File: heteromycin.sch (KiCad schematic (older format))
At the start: 0 parts

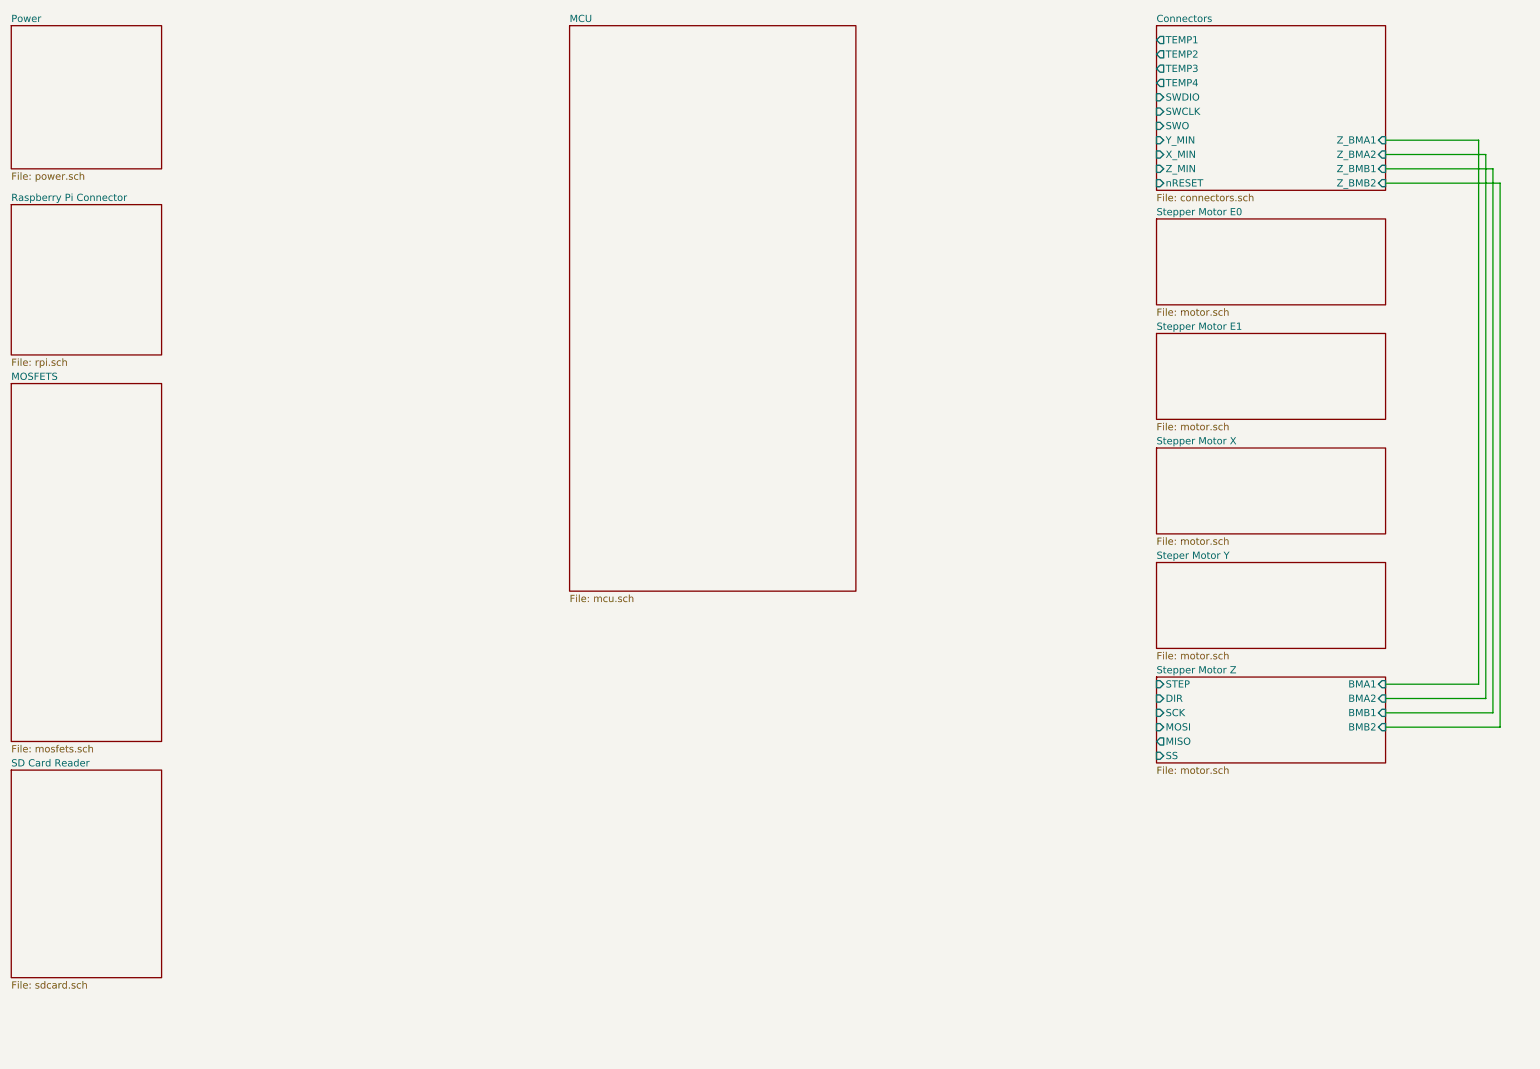
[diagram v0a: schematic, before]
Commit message: Some small adjustments
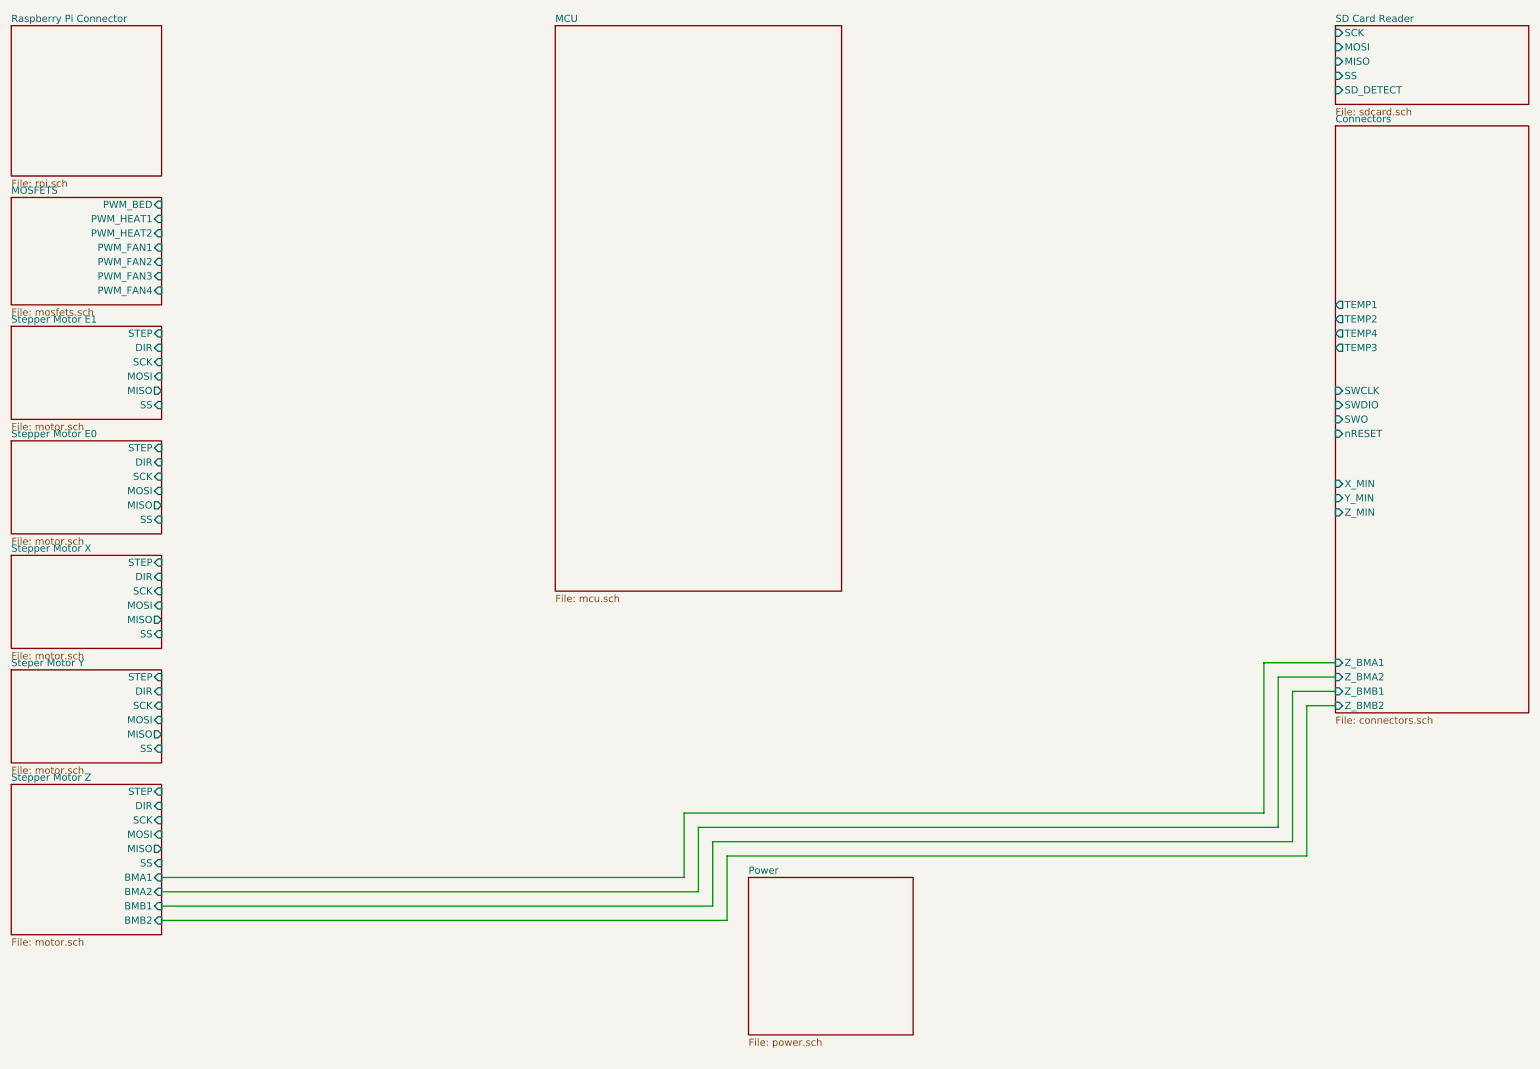
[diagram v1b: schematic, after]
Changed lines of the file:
@@
 $EndDescr
 $Sheet
-S 550  1850 1050 1050
+S 550  600  1050 1050
 U 5BC4AC32
 F0 "Raspberry Pi Connector" 50
@@
 $EndSheet
 $Sheet
-S 550  600  1050 1000
+S 5700 6550 1150 1100
 U 5BC54251
 F0 "Power" 50
@@
 $EndSheet
 $Sheet
-S 4450 600  2000 3950
+S 4350 600  2000 3950
 U 5BC1C8A4
 F0 "MCU" 50
@@
 $EndSheet
 $Sheet
-S 8550 600  1600 1150
+S 550  4300 1050 650
+U 5BC2F52C
+F0 "Stepper Motor X" 50
+F1 "motor.sch" 50
+F2 "STEP" I R 1600 4350 50
+F3 "DIR" I R 1600 4450 50
+F4 "SCK" I R 1600 4550 50
+F5 "MOSI" I R 1600 4650 50
+F6 "MISO" O R 1600 4750 50
+F7 "SS" I R 1600 4850 50
+$EndSheet
+$Sheet
+S 550  1800 1050 750
+U 5BC2F648
+F0 "MOSFETS" 50
+F1 "mosfets.sch" 50
+F2 "PWM_BED" I R 1600 1850 50
+F3 "PWM_HEAT1" I R 1600 1950 50
+F4 "PWM_FAN1" I R 1600 2150 50
+F5 "PWM_FAN3" I R 1600 2350 50
+F6 "PWM_HEAT2" I R 1600 2050 50
+F7 "PWM_FAN2" I R 1600 2250 50
+F8 "PWM_FAN4" I R 1600 2450 50
+$EndSheet
+$Sheet
+S 550  5100 1050 650
+U 5BC77BE8
+F0 "Steper Motor Y" 50
+F1 "motor.sch" 50
+F2 "STEP" I R 1600 5150 50
+F3 "DIR" I R 1600 5250 50
+F4 "SCK" I R 1600 5350 50
+F5 "MOSI" I R 1600 5450 50
+F6 "MISO" O R 1600 5550 50
+F7 "SS" I R 1600 5650 50
+$EndSheet
+$Sheet
+S 550  5900 1050 1050
+U 5BC77F87
+F0 "Stepper Motor Z" 50
+F1 "motor.sch" 50
+F2 "STEP" I R 1600 5950 50
+F3 "DIR" I R 1600 6050 50
+F4 "SCK" I R 1600 6150 50
+F5 "MOSI" I R 1600 6250 50
+F6 "MISO" O R 1600 6350 50
+F7 "BMA1" I R 1600 6550 50
+F8 "BMA2" I R 1600 6650 50
+F9 "BMB2" I R 1600 6850 50
+F10 "BMB1" I R 1600 6750 50
+F11 "SS" I R 1600 6450 50
+$EndSheet
+$Sheet
+S 550  3500 1050 650
+U 5BC77F8A
+F0 "Stepper Motor E0" 50
+F1 "motor.sch" 50
+F2 "STEP" I R 1600 3550 50
+F3 "DIR" I R 1600 3650 50
+F4 "SCK" I R 1600 3750 50
+F5 "MOSI" I R 1600 3850 50
+F6 "MISO" O R 1600 3950 50
+F7 "SS" I R 1600 4050 50
+$EndSheet
+$Sheet
+S 550  2700 1050 650
+U 5BC77F8D
+F0 "Stepper Motor E1" 50
+F1 "motor.sch" 50
+F2 "STEP" I R 1600 2750 50
+F3 "DIR" I R 1600 2850 50
+F4 "SCK" I R 1600 2950 50
+F5 "MOSI" I R 1600 3050 50
+F6 "MISO" O R 1600 3150 50
+F7 "SS" I R 1600 3250 50
+$EndSheet
+$Sheet
+S 9800 600  1350 550
+U 5BC78E83
+F0 "SD Card Reader" 50
+F1 "sdcard.sch" 50
+F2 "MISO" I L 9800 850 50
+F3 "MOSI" I L 9800 750 50
+F4 "SCK" I L 9800 650 50
+F5 "SD_DETECT" I L 9800 1050 50
+F6 "SS" I L 9800 950 50
+$EndSheet
+$Sheet
+S 9800 1300 1350 4100
 U 5BC2F290
 F0 "Connectors" 50
 F1 "connectors.sch" 50
-F2 "TEMP1" O L 8550 700 50
-F3 "TEMP2" O L 8550 800 50
-F4 "TEMP3" O L 8550 900 50
-F5 "nRESET" I L 8550 1700 50
-F6 "SWDIO" I L 8550 1100 50
-F7 "SWCLK" I L 8550 1200 50
-F8 "Z_MIN" I L 8550 1600 50
-F9 "Y_MIN" I L 8550 1400 50
-F10 "Z_BMB1" I R 10150 1600 50
-F11 "Z_BMB2" I R 10150 1700 50
-F12 "Z_BMA2" I R 10150 1500 50
-F13 "Z_BMA1" I R 10150 1400 50
-F14 "X_MIN" I L 8550 1500 50
-F15 "SWO" I L 8550 1300 50
-F16 "TEMP4" O L 8550 1000 50
-$EndSheet
-$Sheet
-S 8550 3550 1600 600
-U 5BC2F52C
-F0 "Stepper Motor X" 50
-F1 "motor.sch" 50
-$EndSheet
-$Sheet
-S 550  3100 1050 2500
-U 5BC2F648
-F0 "MOSFETS" 50
-F1 "mosfets.sch" 50
-$EndSheet
-$Sheet
-S 8550 4350 1600 600
-U 5BC77BE8
-F0 "Steper Motor Y" 50
-F1 "motor.sch" 50
-$EndSheet
-$Sheet
-S 8550 5150 1600 600
-U 5BC77F87
-F0 "Stepper Motor Z" 50
-F1 "motor.sch" 50
-F2 "STEP" I L 8550 5200 50
-F3 "DIR" I L 8550 5300 50
-F4 "SCK" I L 8550 5400 50
-F5 "MOSI" I L 8550 5500 50
-F6 "MISO" O L 8550 5600 50
-F7 "BMA1" I R 10150 5200 50
-F8 "BMA2" I R 10150 5300 50
-F9 "BMB2" I R 10150 5500 50
-F10 "BMB1" I R 10150 5400 50
-F11 "SS" I L 8550 5700 50
-$EndSheet
-$Sheet
-S 8550 1950 1600 600
-U 5BC77F8A
-F0 "Stepper Motor E0" 50
-F1 "motor.sch" 50
-$EndSheet
-$Sheet
-S 8550 2750 1600 600
-U 5BC77F8D
-F0 "Stepper Motor E1" 50
-F1 "motor.sch" 50
+F2 "Z_BMB1" I L 9800 5250 50
+F3 "Z_BMB2" I L 9800 5350 50
+F4 "Z_BMA2" I L 9800 5150 50
+F5 "Z_BMA1" I L 9800 5050 50
+F6 "TEMP1" O L 9800 2550 50
+F7 "TEMP2" O L 9800 2650 50
+F8 "TEMP3" O L 9800 2850 50
+F9 "nRESET" I L 9800 3450 50
+F10 "SWDIO" I L 9800 3250 50
+F11 "SWCLK" I L 9800 3150 50
+F12 "Z_MIN" I L 9800 4000 50
+F13 "Y_MIN" I L 9800 3900 50
+F14 "X_MIN" I L 9800 3800 50
+F15 "SWO" I L 9800 3350 50
+F16 "TEMP4" O L 9800 2750 50
 $EndSheet
 Wire Wire Line
-	10150 5200 10800 5200
+	1600 6850 5550 6850
 Wire Wire Line
-	10800 5200 10800 1400
+	5550 6850 5550 6400
 Wire Wire Line
-	10800 1400 10150 1400
+	5550 6400 9600 6400
 Wire Wire Line
-	10150 1500 10850 1500
+	9600 6400 9600 5350
 Wire Wire Line
-	10850 1500 10850 5300
+	9600 5350 9800 5350
 Wire Wire Line
-	10850 5300 10150 5300
+	9800 5250 9500 5250
 Wire Wire Line
-	10150 5400 10900 5400
+	9500 5250 9500 6300
 Wire Wire Line
-	10900 5400 10900 1600
+	9500 6300 5450 6300
 Wire Wire Line
-	10900 1600 10150 1600
+	5450 6300 5450 6750
 Wire Wire Line
-	10150 1700 10950 1700
+	5450 6750 1600 6750
 Wire Wire Line
-	10950 1700 10950 5500
+	1600 6650 5350 6650
 Wire Wire Line
-	10950 5500 10150 5500
-$Sheet
-S 550  5800 1050 1450
-U 5BC78E83
-F0 "SD Card Reader" 50
-F1 "sdcard.sch" 50
-$EndSheet
+	5350 6650 5350 6200
+Wire Wire Line
+	5350 6200 9400 6200
+Wire Wire Line
+	9400 6200 9400 5150
+Wire Wire Line
+	9400 5150 9800 5150
+Wire Wire Line
+	9800 5050 9300 5050
+Wire Wire Line
+	9300 5050 9300 6100
+Wire Wire Line
+	9300 6100 5250 6100
+Wire Wire Line
+	5250 6100 5250 6550
+Wire Wire Line
+	5250 6550 1600 6550
 $EndSCHEMATC

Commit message: First pass of routing
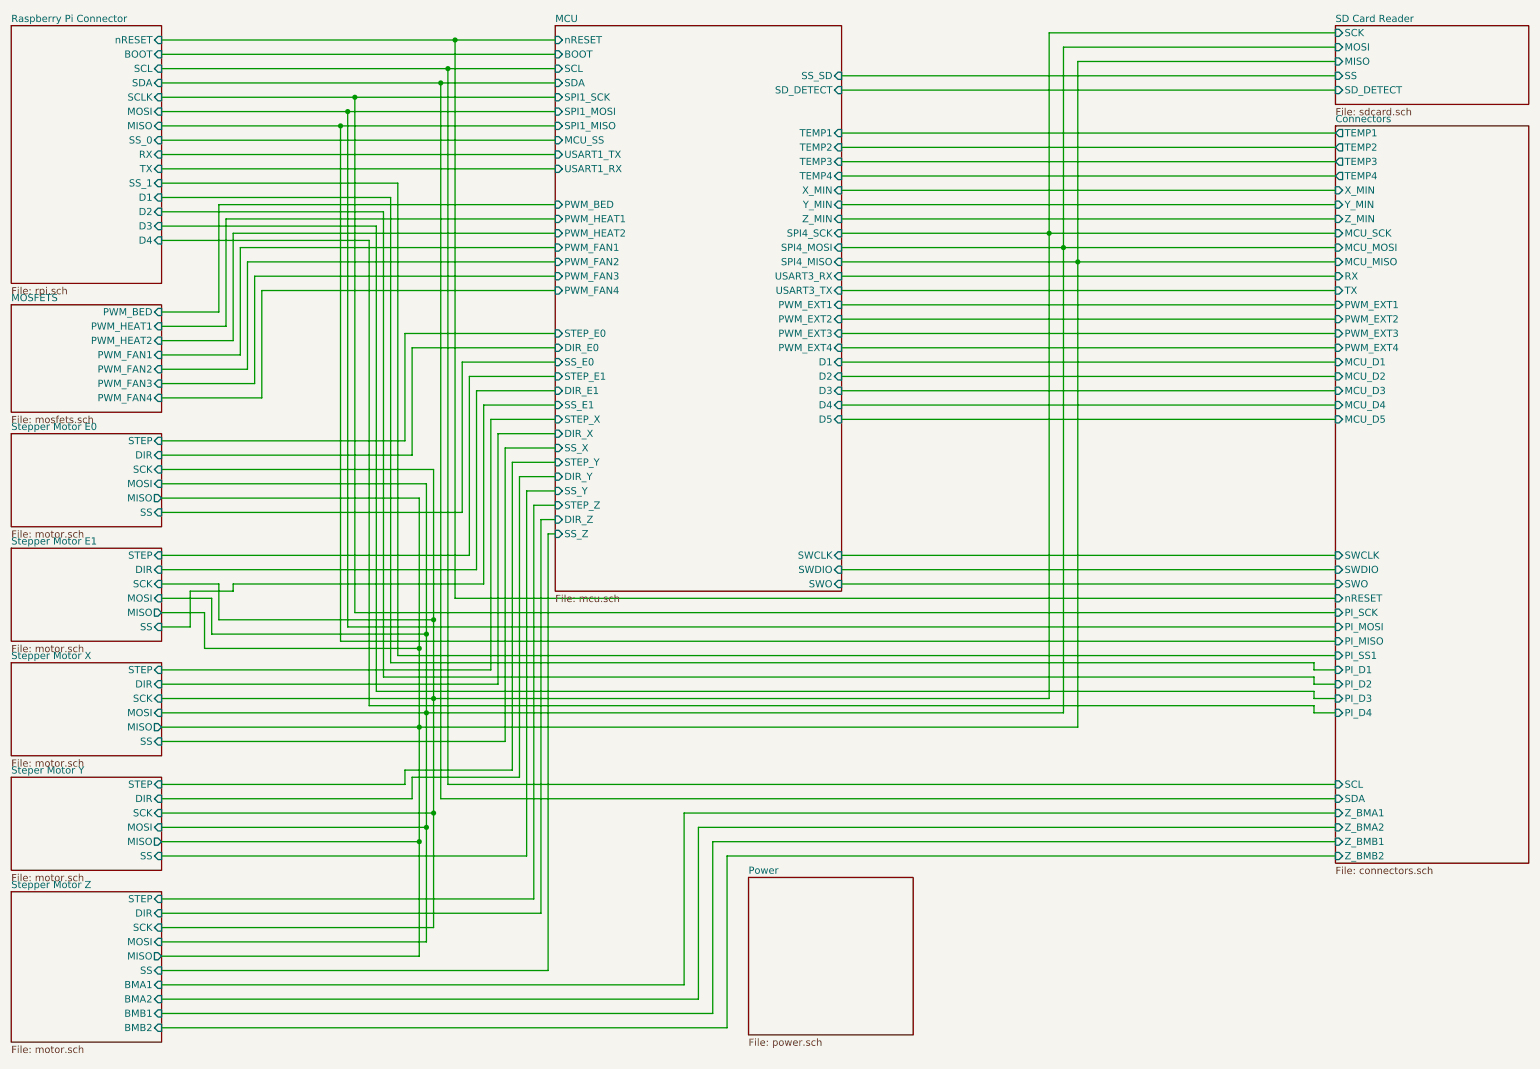
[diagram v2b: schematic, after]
